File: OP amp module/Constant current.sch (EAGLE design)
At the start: 8 parts, among them IC1 LM358N

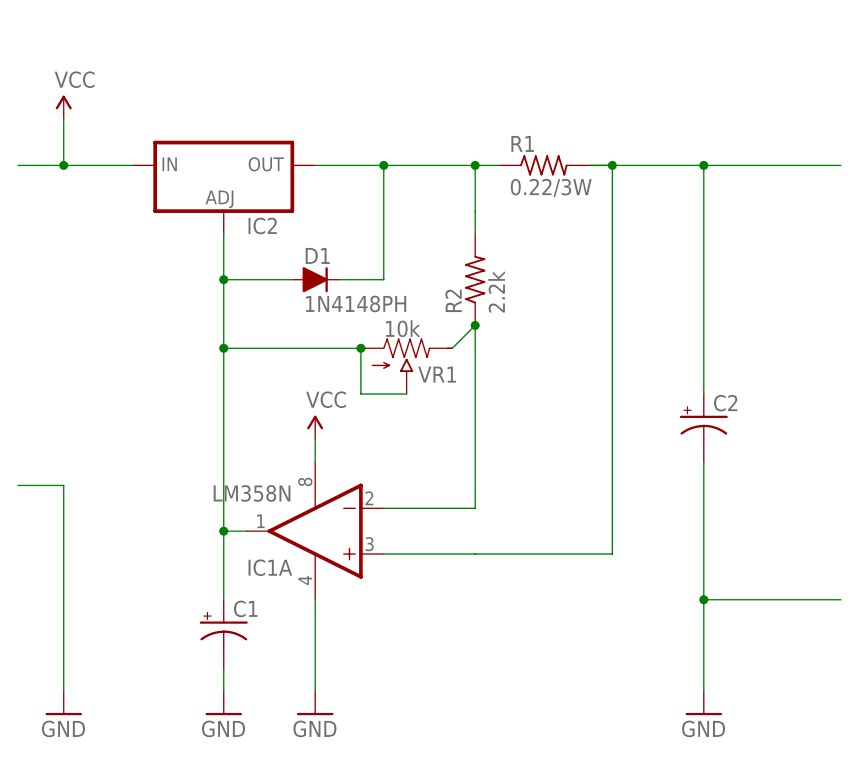
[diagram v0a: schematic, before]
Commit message: My Library
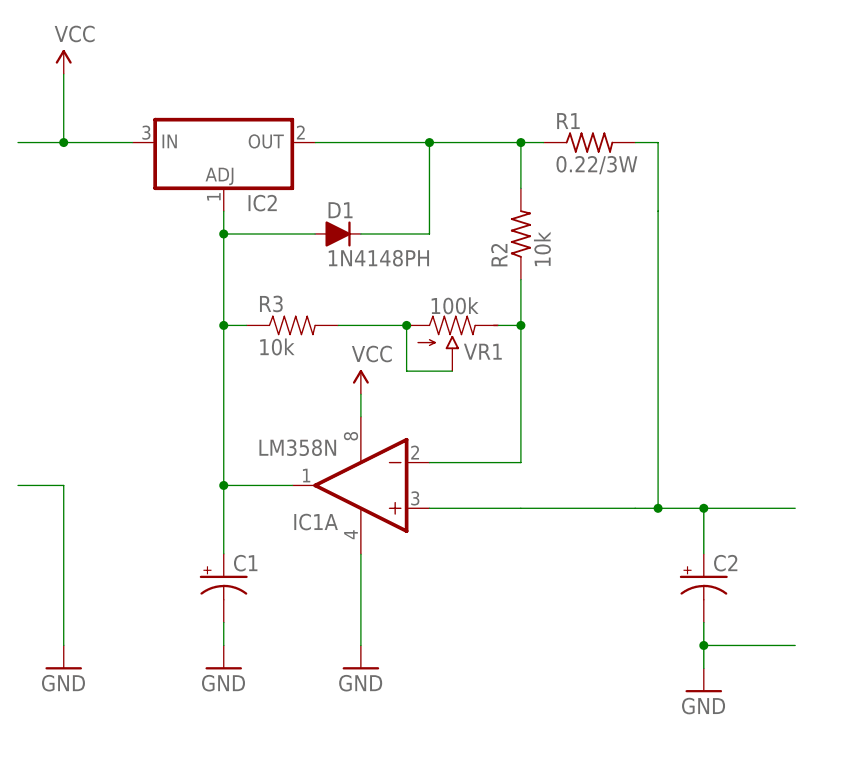
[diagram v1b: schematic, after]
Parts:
- added R3: 10k, SparkFun:RESISTORKIT
- R2: value 2.2k -> 10k
- VR1: value 10k -> 100k
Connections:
- new net N$4: R3.2, VR1.A, VR1.S
- net N$2: now also R3.1; no longer VR1.A, VR1.S
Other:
- moved on the sheet: C1, C2, D1, IC1A, R1, R2, VR1
